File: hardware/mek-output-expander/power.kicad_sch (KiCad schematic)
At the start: 25 parts, among them U1 LMR38020FDDAR, U2 AMS1117-3.3

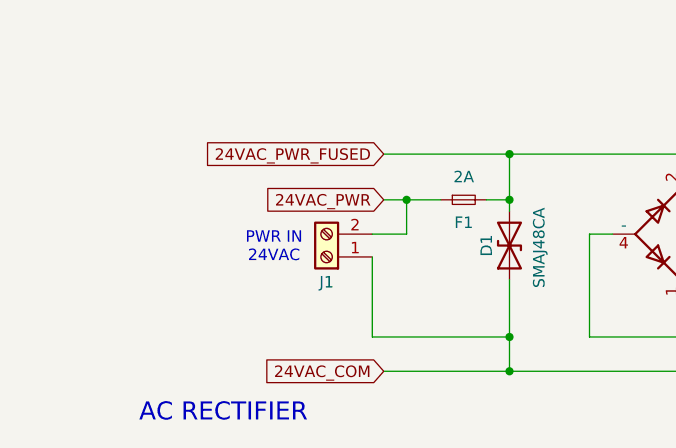
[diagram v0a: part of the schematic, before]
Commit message: Updates
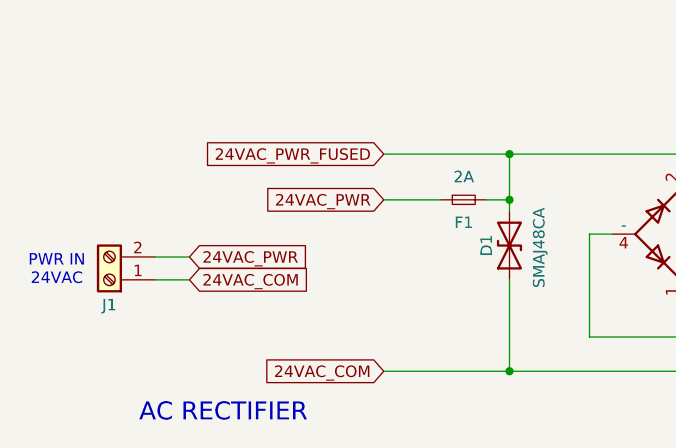
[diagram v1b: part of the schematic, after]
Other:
- moved on the sheet: J1
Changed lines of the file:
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@@
 	(text "PWR IN\n24VAC\n"
 		(exclude_from_sim no)
-		(at 47.498 172.974 0)
+		(at 23.368 175.514 0)
 		(effects
 			(font
@@
 	)
 	(junction
-		(at 73.66 182.88)
-		(diameter 0)
-		(color 0 0 0 0)
-	)
-	(junction
 		(at 162.56 119.38)
 		(diameter 0)
@@
 	)
 	(junction
-		(at 62.23 167.64)
-		(diameter 0)
-		(color 0 0 0 0)
-	)
-	(junction
 		(at 134.62 93.98)
 		(diameter 0)
@@
 	(wire
 		(pts
-			(xy 59.69 167.64) (xy 62.23 167.64)
-		)
-		(stroke
-			(width 0)
-			(type default)
-		)
-	)
-	(wire
-		(pts
-			(xy 73.66 176.53) (xy 73.66 182.88)
+			(xy 59.69 167.64) (xy 66.04 167.64)
+		)
+		(stroke
+			(width 0)
+			(type default)
+		)
+	)
+	(wire
+		(pts
+			(xy 73.66 176.53) (xy 73.66 186.69)
 		)
 		(stroke
@@
 	(wire
 		(pts
-			(xy 62.23 171.45) (xy 62.23 167.64)
-		)
-		(stroke
-			(width 0)
-			(type default)
-		)
-	)
-	(wire
-		(pts
 			(xy 69.85 40.64) (xy 77.47 40.64)
 		)
@@
 	(wire
 		(pts
-			(xy 58.42 171.45) (xy 62.23 171.45)
-		)
-		(stroke
-			(width 0)
-			(type default)
-		)
-	)
-	(wire
-		(pts
 			(xy 58.42 86.36) (xy 64.77 86.36)
 		)
@@
 	(wire
 		(pts
-			(xy 58.42 182.88) (xy 73.66 182.88)
-		)
-		(stroke
-			(width 0)
-			(type default)
-		)
-	)
-	(wire
-		(pts
 			(xy 82.55 171.45) (xy 82.55 182.88)
 		)
@@
 	(wire
 		(pts
+			(xy 34.29 173.99) (xy 38.1 173.99)
+		)
+		(stroke
+			(width 0)
+			(type default)
+		)
+	)
+	(wire
+		(pts
 			(xy 162.56 93.98) (xy 166.37 93.98)
 		)
@@
 	(wire
 		(pts
+			(xy 34.29 176.53) (xy 38.1 176.53)
+		)
+		(stroke
+			(width 0)
+			(type default)
+		)
+	)
+	(wire
+		(pts
 			(xy 85.09 171.45) (xy 82.55 171.45)
 		)
@@
 	(wire
 		(pts
-			(xy 62.23 167.64) (xy 66.04 167.64)
-		)
-		(stroke
-			(width 0)
-			(type default)
-		)
-	)
-	(wire
-		(pts
-			(xy 58.42 182.88) (xy 58.42 173.99)
-		)
-		(stroke
-			(width 0)
-			(type default)
-		)
-	)
-	(wire
-		(pts
 			(xy 134.62 93.98) (xy 134.62 100.33)
 		)
@@
 		(pts
 			(xy 226.06 157.48) (xy 220.98 157.48)
-		)
-		(stroke
-			(width 0)
-			(type default)
-		)
-	)
-	(wire
-		(pts
-			(xy 73.66 186.69) (xy 73.66 182.88)
 		)
 		(stroke
@@
 		)
 	)
+	(global_label "24VAC_PWR"
+		(shape input)
+		(at 38.1 173.99 0)
+		(fields_autoplaced yes)
+		(effects
+			(font
+				(size 1.27 1.27)
+			)
+			(justify left)
+		)
+		(property "Intersheetrefs" "${INTERSHEET_REFS}"
+			(at 51.9104 173.99 0)
+			(hide yes)
+			(show_name no)
+			(do_not_autoplace no)
+			(effects
+				(font
+					(size 1.27 1.27)
+				)
+				(justify left)
+			)
+		)
+	)
 	(global_label "GND"
 		(shape input)
@@
 		(property "Intersheetrefs" "${INTERSHEET_REFS}"
 			(at 173.2257 119.38 0)
+			(hide yes)
+			(show_name no)
+			(do_not_autoplace no)
+			(effects
+				(font
+					(size 1.27 1.27)
+				)
+				(justify left)
+			)
+		)
+	)
+	(global_label "24VAC_COM"
+		(shape input)
+		(at 38.1 176.53 0)
+		(fields_autoplaced yes)
+		(effects
+			(font
+				(size 1.27 1.27)
+			)
+			(justify left)
+		)
+		(property "Intersheetrefs" "${INTERSHEET_REFS}"
+			(at 51.9709 176.53 0)
 			(hide yes)
 			(show_name no)
@@
 	(symbol
 		(lib_id "Connector:Screw_Terminal_01x02")
-		(at 53.34 173.99 180)
+		(at 29.21 176.53 180)
 		(unit 1)
 		(body_style 1)
@@
 		(dnp no)
 		(property "Reference" "J1"
-			(at 53.34 176.784 0)
+			(at 29.21 179.324 0)
 			(show_name no)
 			(do_not_autoplace no)
@@
 		)
 		(property "Value" ""
-			(at 45.72 173.99 0)
+			(at 21.59 176.53 0)
 			(show_name no)
 			(do_not_autoplace no)
@@
 		)
 		(property "Footprint" "TerminalBlock_Phoenix:TerminalBlock_Phoenix_MKDS-1,5-2-5.08_1x02_P5.08mm_Horizontal"
-			(at 53.34 173.99 0)
+			(at 29.21 176.53 0)
 			(hide yes)
 			(show_name no)
@@
 		)
 		(property "Datasheet" ""
-			(at 53.34 173.99 0)
+			(at 29.21 176.53 0)
 			(hide yes)
 			(show_name no)
@@
 		)
 		(property "Description" ""
-			(at 53.34 173.99 0)
+			(at 29.21 176.53 0)
 			(hide yes)
 			(show_name no)
@@
 		)
 		(property "KLC_S3.3" ""
-			(at 53.34 173.99 0)
+			(at 29.21 176.53 0)
 			(hide yes)
 			(show_name no)
@@
 		)
 		(property "KLC_S4.1" ""
-			(at 53.34 173.99 0)
+			(at 29.21 176.53 0)
 			(hide yes)
 			(show_name no)
@@
 		)
 		(property "LCSC Part #" "N/A"
-			(at 53.34 173.99 0)
-			(hide yes)
-			(show_name no)
+			(at 29.21 176.53 0)
+			(hide yes)
+			(show_name no)
